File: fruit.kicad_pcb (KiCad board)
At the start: 4 copper layers, 161.6 x 100 mm, 178 parts, among them J1 PCB_Edge_PCI_Express_x4_Salmo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, J2 2086581051, J3 TSM-102-01-L-SV, J4 TSM-102-01-L-SV, J5 MEM2067-02-180-00-A_REVB, J6 USB4110-GF-A, J7 USB4110-GF-A, J8 1-2199119-6, U1 INA260, U10 LM3525M-H_NPOB, U11 USB3740B-AI2, U12 AP22653FDZ-7, U13 AP64501SP-13, U14 AP64501SP-13, U2 PCA9671BS,118, U3 PCA9671BS,118, U4 AP22653FDZ-7, U5 TPD8S009DSMR, U6 INA260, U7 MCP9808T-E_MC, U8 ADS7142IRUGR, U9 MCP9808T-E_MC

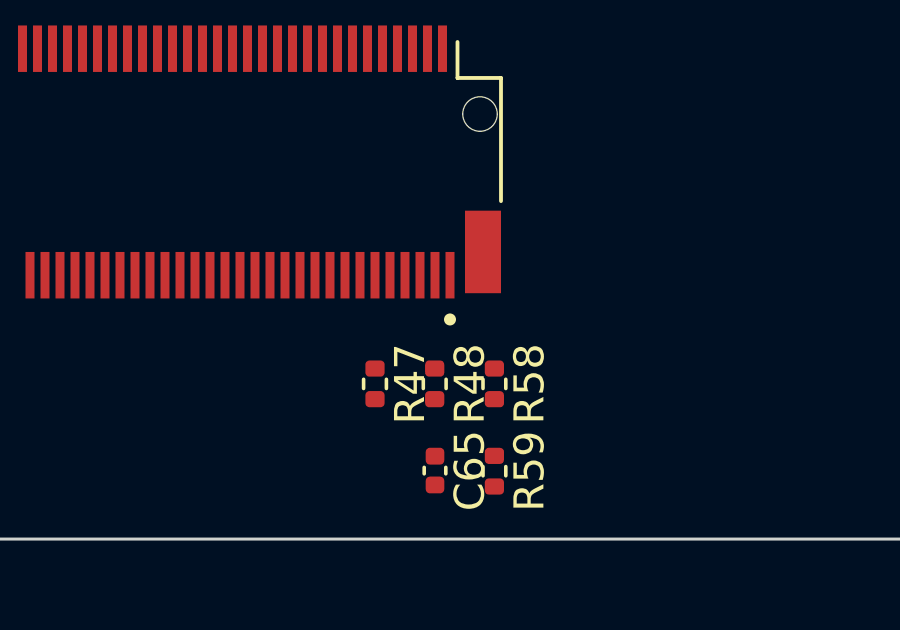
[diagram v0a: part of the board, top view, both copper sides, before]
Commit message: locked cm4 & mech footprints
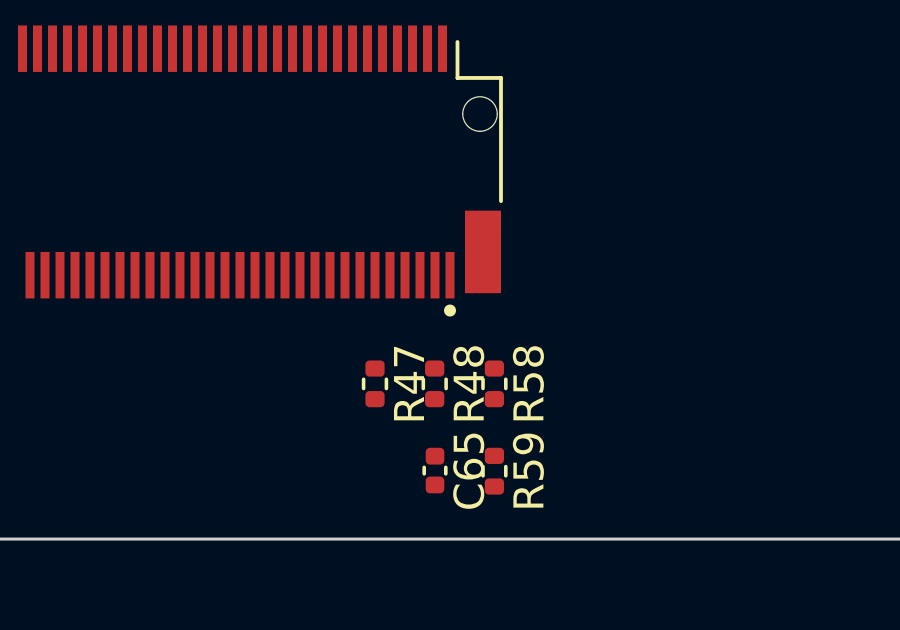
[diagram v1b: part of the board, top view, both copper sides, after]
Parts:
- COOLER1: value 53-61mm_NorthBridge_45deg_arms -> 53-61
- J2: value 2086581051 -> CONN_208658-1051_MOL
- J6, J7: value USB4110-GF-A -> GCT_USB4110-GF-A
- U8: value ADS7142IRUGR -> RUG0010A
